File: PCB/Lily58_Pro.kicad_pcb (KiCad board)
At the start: 2 copper layers, 142.5 x 106.3 mm, 128 parts, among them J1 LED, J2 4PIN, J3 OLED, P1 i2c_pin, P2 i2c_pin, SW1 SW_PUSH, SW10 SW_PUSH, SW11 SW_PUSH, SW12 SW_PUSH, SW13 SW_PUSH, SW14 SW_PUSH, SW15 SW_PUSH, SW16 SW_PUSH, SW17 SW_PUSH, SW18 SW_PUSH, SW19 SW_PUSH, SW2 SW_PUSH, SW20 SW_PUSH, SW21 SW_PUSH, SW22 SW_PUSH, SW23 SW_PUSH, SW24 SW_PUSH, SW25 Rotary_Encoder_Switch, SW26 SW_PUSH, SW27 SW_PUSH, SW28 SW_PUSH, SW29 SW_PUSH, SW3 SW_PUSH, SW4 SW_PUSH, SW5 SW_PUSH, SW6 SW_PUSH, SW7 SW_PUSH, SW8 SW_PUSH, SW9 SW_PUSH, U1 ProMicro

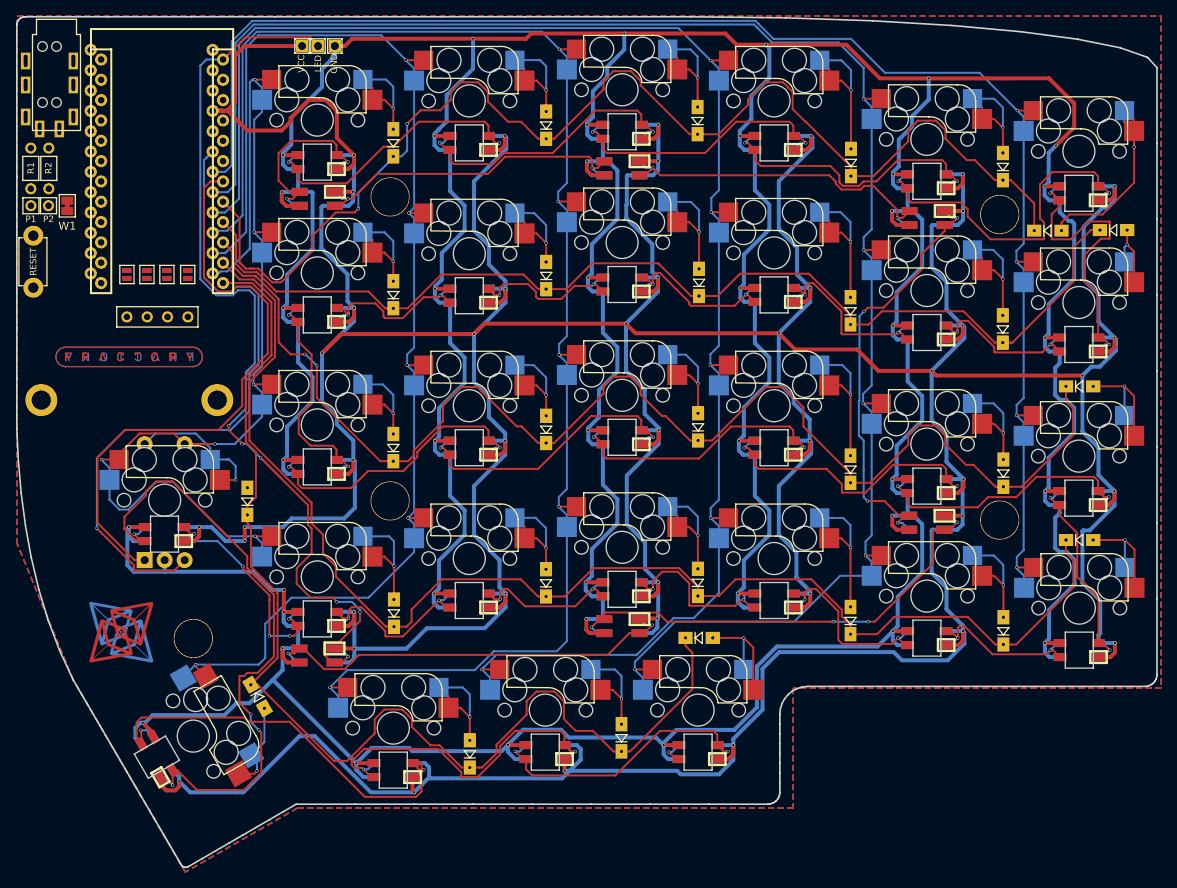
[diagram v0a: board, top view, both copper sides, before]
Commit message: Net done
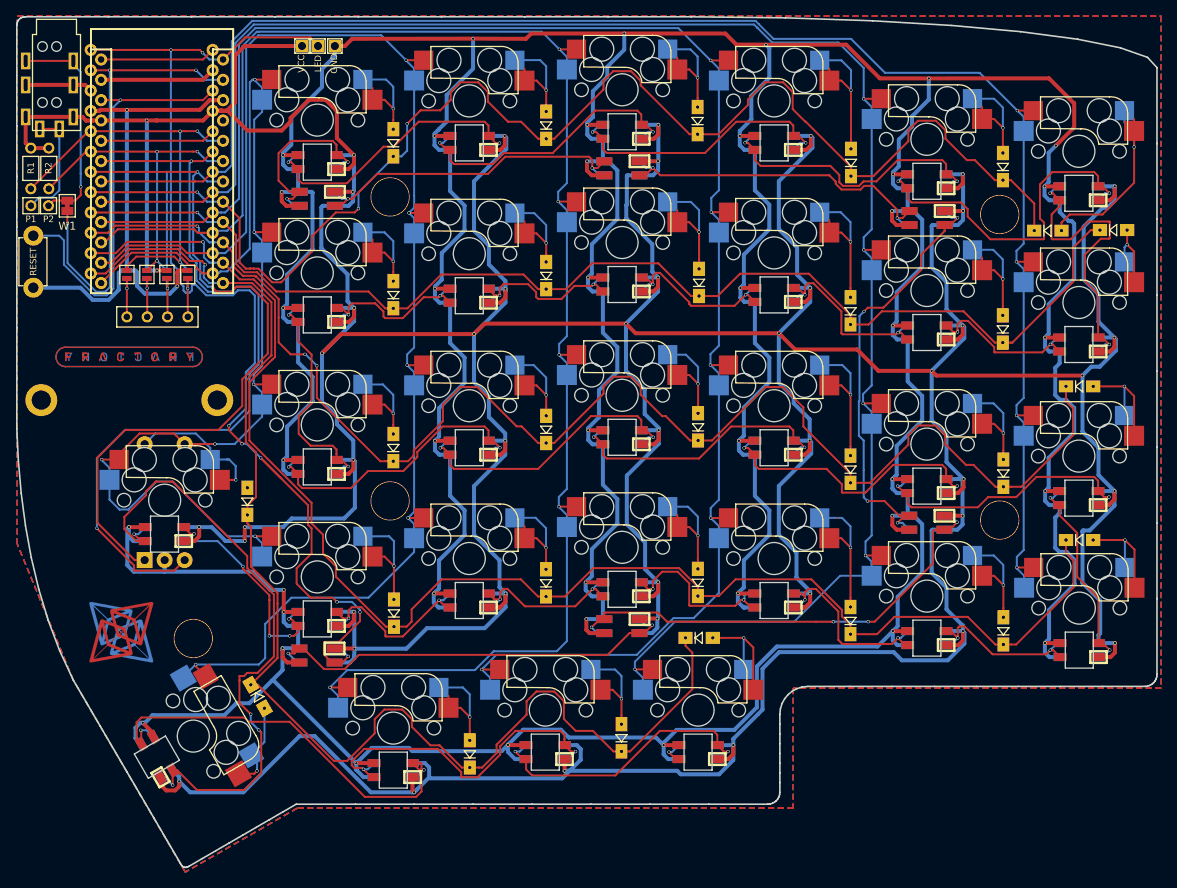
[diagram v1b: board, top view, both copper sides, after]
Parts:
- renumbered G*** to G1, G*** to G10, G*** to G11, G*** to G12, G*** to G13, G*** to G2, G*** to G3, G*** to G4, G*** to G5, G*** to G6
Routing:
- net GND: track 856.6 -> 943.7 mm, vias 41 -> 43
- net DATA: track 0.00 -> 57.7 mm, vias 0 -> 3
- net SCL: track 0.00 -> 53.8 mm, vias 0 -> 3
- net RESET: track 0.00 -> 53.6 mm, vias 0 -> 1
- net SDA: track 0.00 -> 53.3 mm, vias 0 -> 3
- net VCC: track 899.6 -> 951.3 mm, vias 43 -> 45
- net Net-(J2-Pad3): track 0.00 -> 27.7 mm, vias 0 -> 1
- net row4: track 147.0 -> 167.8 mm, vias 0 -> 1
- net LED: track 121.8 -> 142.4 mm, vias 6 -> 8
- net row3: track 167.8 -> 187.1 mm, vias 0 -> 1
- net row2: track 166.7 -> 184.8 mm, vias 2 -> 3
- net enc1: track 74.7 -> 92.1 mm, vias 0 -> 2
- net row1: track 136.8 -> 153.8 mm, vias 0 -> 1
- net row0: track 157.3 -> 174.3 mm, vias 2 -> 3
- net col5: track 135.4 -> 152.0 mm
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
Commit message: Finishing
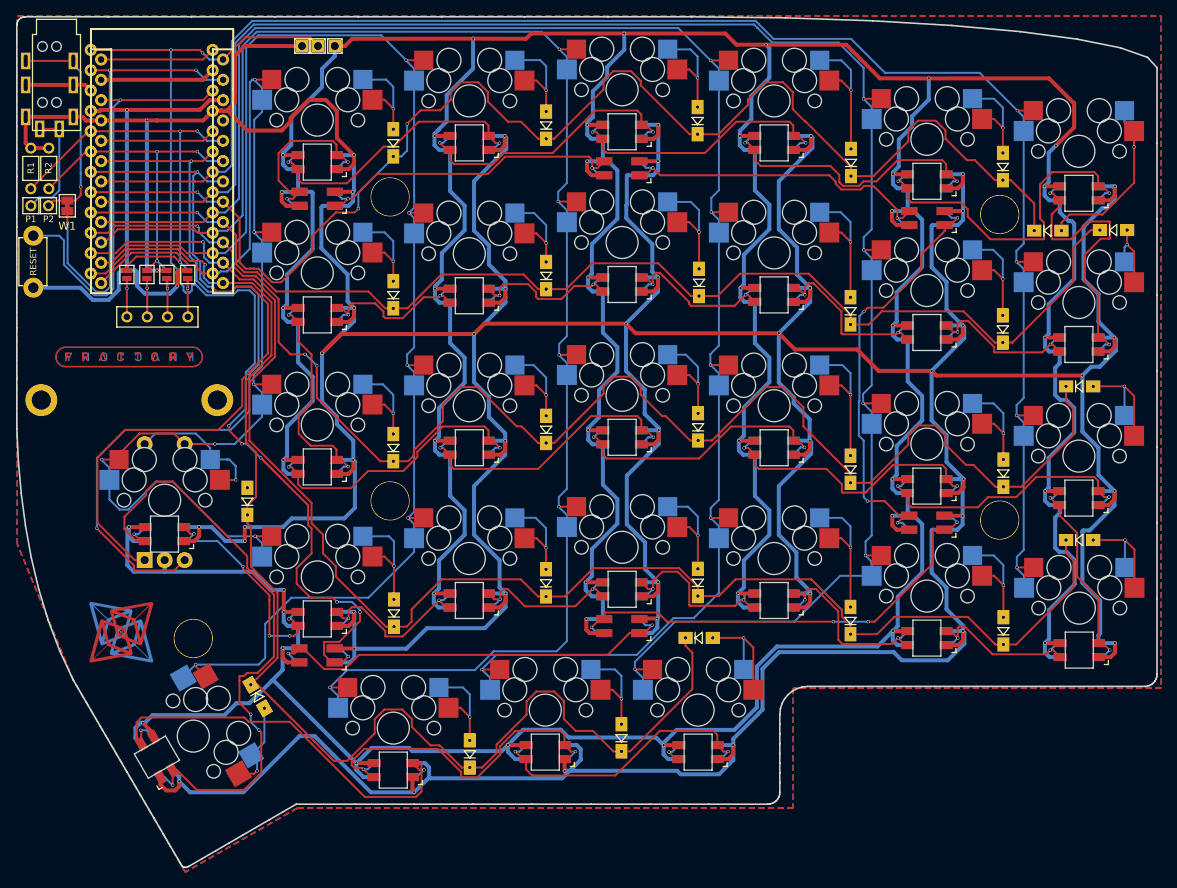
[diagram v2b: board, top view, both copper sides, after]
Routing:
- net SCL: track 53.8 -> 41.4 mm
- net Net-(D7-Pad2): track 14.0 -> 12.3 mm
- net Net-(D11-Pad2): track 15.9 -> 14.3 mm
- net Net-(D10-Pad2): track 18.5 -> 16.9 mm
- net Net-(D9-Pad2): track 16.4 -> 14.9 mm
- net Net-(D8-Pad2): track 13.9 -> 12.4 mm
- net Net-(D6-Pad2): track 25.2 -> 23.7 mm
- net Net-(D5-Pad2): track 14.5 -> 13.0 mm
- net Net-(D4-Pad2): track 19.0 -> 17.5 mm
- net Net-(D3-Pad2): track 14.9 -> 13.4 mm
- net Net-(D27-Pad2): track 14.6 -> 13.1 mm
- net Net-(D21-Pad2): track 15.3 -> 13.8 mm
- net Net-(D20-Pad2): track 14.3 -> 12.8 mm
- net Net-(D2-Pad2): track 14.6 -> 13.1 mm
- net Net-(D1-Pad2): track 14.0 -> 12.5 mm
